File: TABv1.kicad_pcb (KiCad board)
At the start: 4 copper layers, 90 x 45 mm, 127 parts, among them IC1 TPS630702RNMR, J1 USB_C_Receptacle_USB2.0_16P, J10 Conn_02x03_Odd_Even, J11 Conn_UART_1, J15 DB141R-2.54-8P-GN, J4 Conn_Coaxial, J5 Conn_02x06_Counter_Clockwise, J6 SWD, J7 503398-1892, J8 1053141104, J9 Conn_02x03_Odd_Even, Q1 MJD44H11T4G, Q10 PJM09P30DF, Q11 PJM09P30DF, Q12 PJM09P30DF, Q13 PJM09P30DF, Q2 NMOS, Q5 NMOS, Q6 NMOS, Q7 NMOS, Q8 NMOS, Q9 NMOS, SW1 BOOTSEL, SW2 RESET, U1 RP2350B-QFN80, U10 RAK3172, U11 LPS22DF, U2 W25Q128JVS, U4 LSM6DSO32TR, U6 LT3092xST, U7 LSM6DSO32TR, U8 LIS2MDL, U9 TESEO-LIV4F, Y1 12MHz

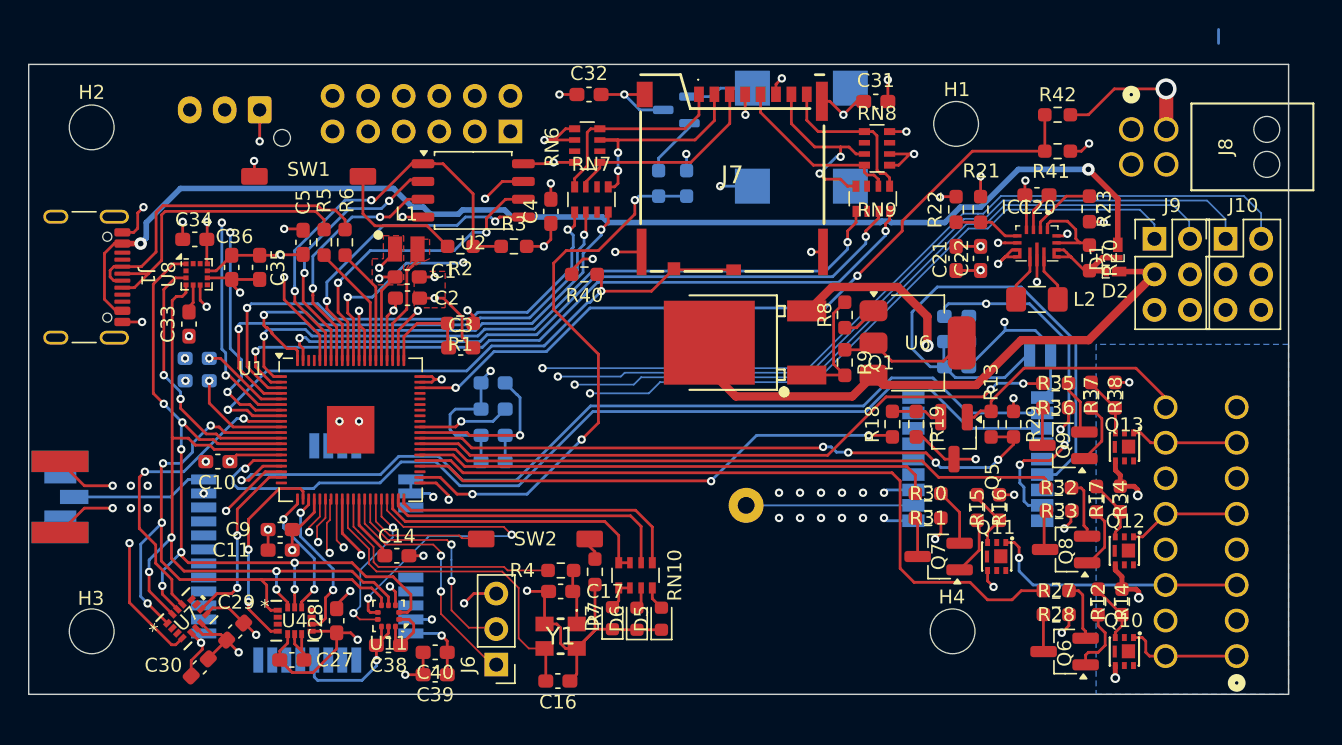
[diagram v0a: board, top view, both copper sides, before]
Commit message: small
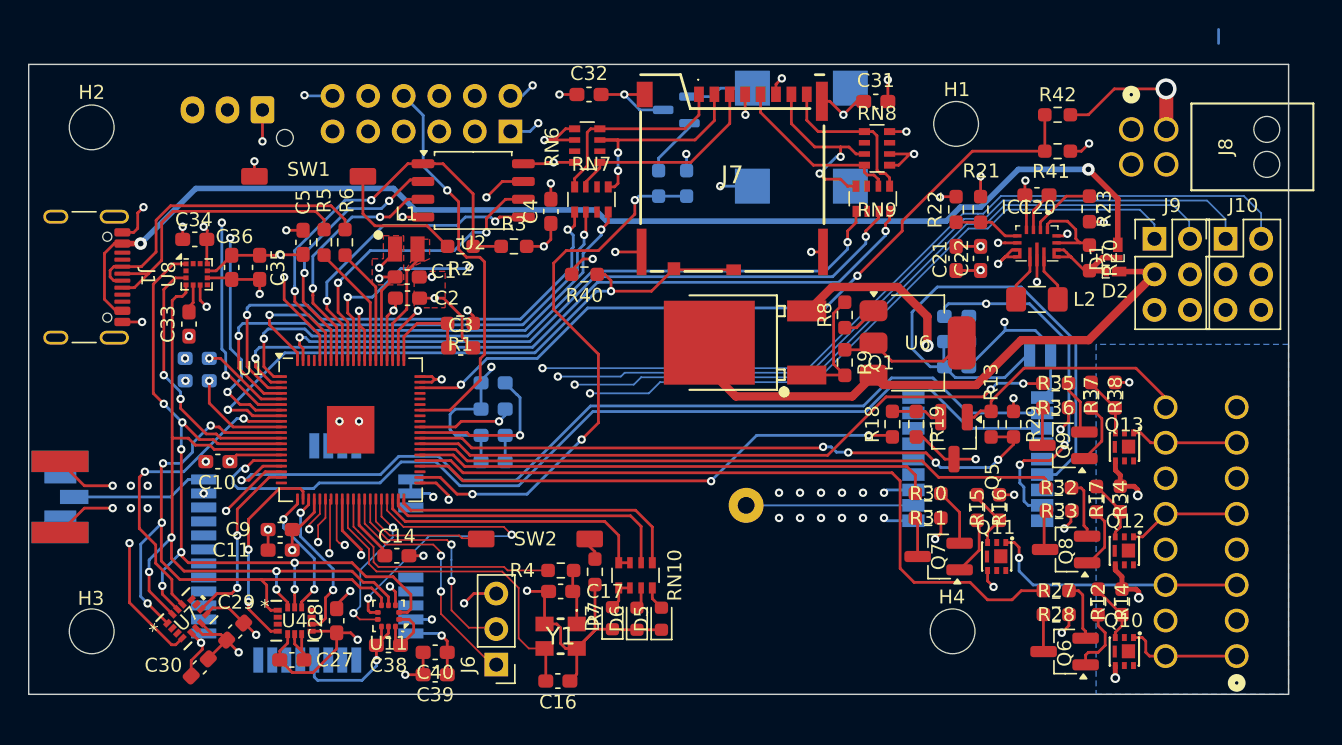
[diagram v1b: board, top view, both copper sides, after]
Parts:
- moved J11 0.20 mm to (89.2, 36.8)
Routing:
- net /GPIO43: track 0.00 -> 28.6 mm, vias 0 -> 1
- net GND: track 165.6 -> 169.4 mm, vias 70 -> 72
- net +3V3: track 157.9 -> 159.6 mm, vias 34 -> 35
- net /SD_CMD: track 33.5 -> 32.4 mm
- net VUSB: track 86.9 -> 85.9 mm
- net /SD_detect: track 45.7 -> 46.3 mm
